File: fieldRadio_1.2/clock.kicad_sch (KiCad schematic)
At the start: 8 parts, among them J9 Conn_01x02, U8 Si5351A-B-GT, Y2 25MHz

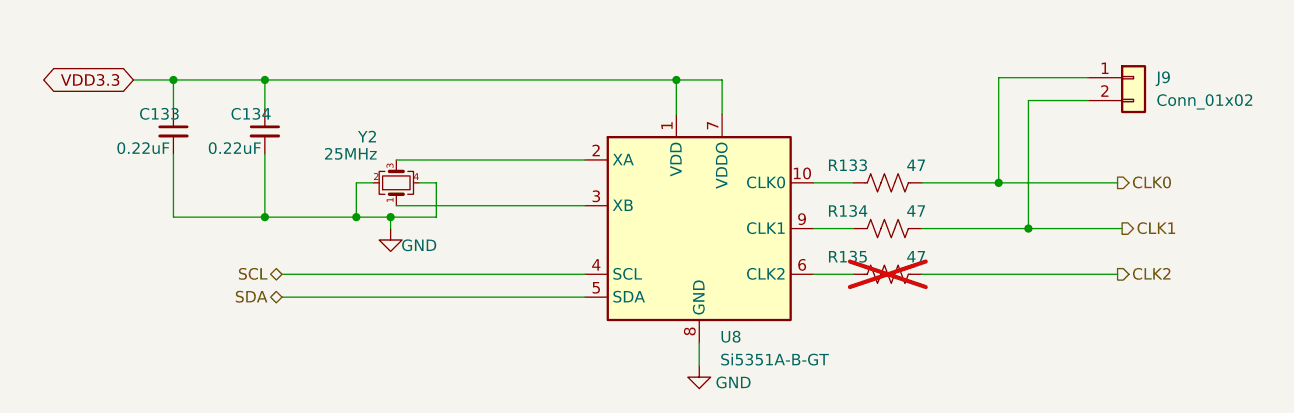
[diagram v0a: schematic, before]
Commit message: updating schematics for fieldRadio_1.2
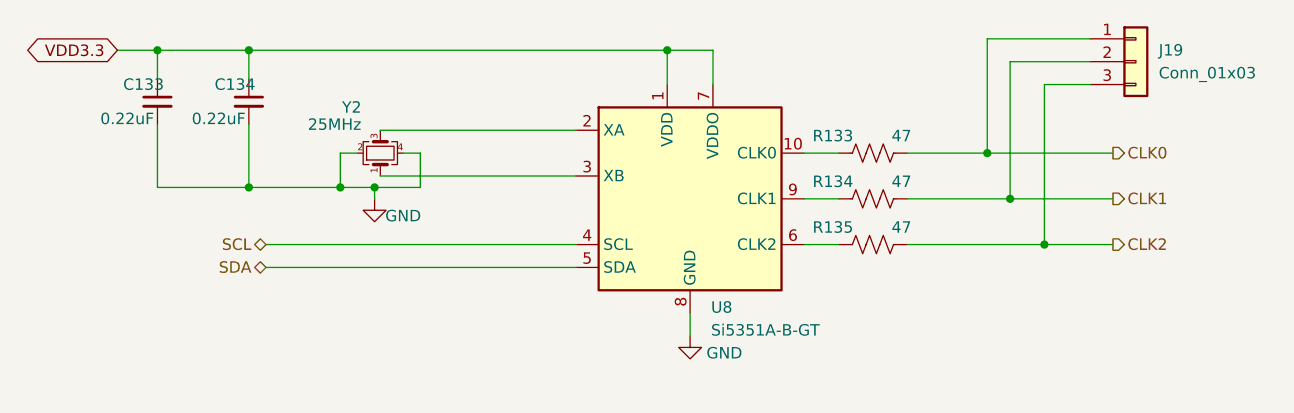
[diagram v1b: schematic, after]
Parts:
- removed J9: Conn_01x02, Connector_PinHeader_2.54mm:PinHeader_1x02_P2.54mm_Vertical, symbol Connector_Generic:Conn_01x02
- added J19: Conn_01x03, Connector_PinHeader_2.54mm:PinHeader_1x03_P2.54mm_Vertical, symbol Connector_Generic:Conn_01x03
- R135: now fitted
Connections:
- net CLK0: now also J19.1 (Pin_1)
- net CLK1: now also J19.2 (Pin_2)
- net CLK2: now also J19.3 (Pin_3)
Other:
- moved on the sheet: C133, C134, R133, R134, U8, Y2
